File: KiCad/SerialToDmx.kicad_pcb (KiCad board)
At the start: 4 copper layers, 158 x 54 mm, 39 parts, among them J1 NAC3MPXXA, J10 Conn_01x08_Pin, J11 Conn_01x08_Pin, J2 NAC3MPXXB, J3 NC3FAV, J4 NC3MAV, J5 NC4FAV, J6 Conn_01x08_Socket, J7 Conn_01x08_Socket, J8 Conn_01x08_Pin, J9 Conn_01x08_Pin, U1 XIAO ESP32 C3, U2 ISOM8710DFFR, U3 ISOM8710DFFR, U4 ISOM8710DFFR, U5 THVD1512DGS, U6 SN74LV1T34DBV

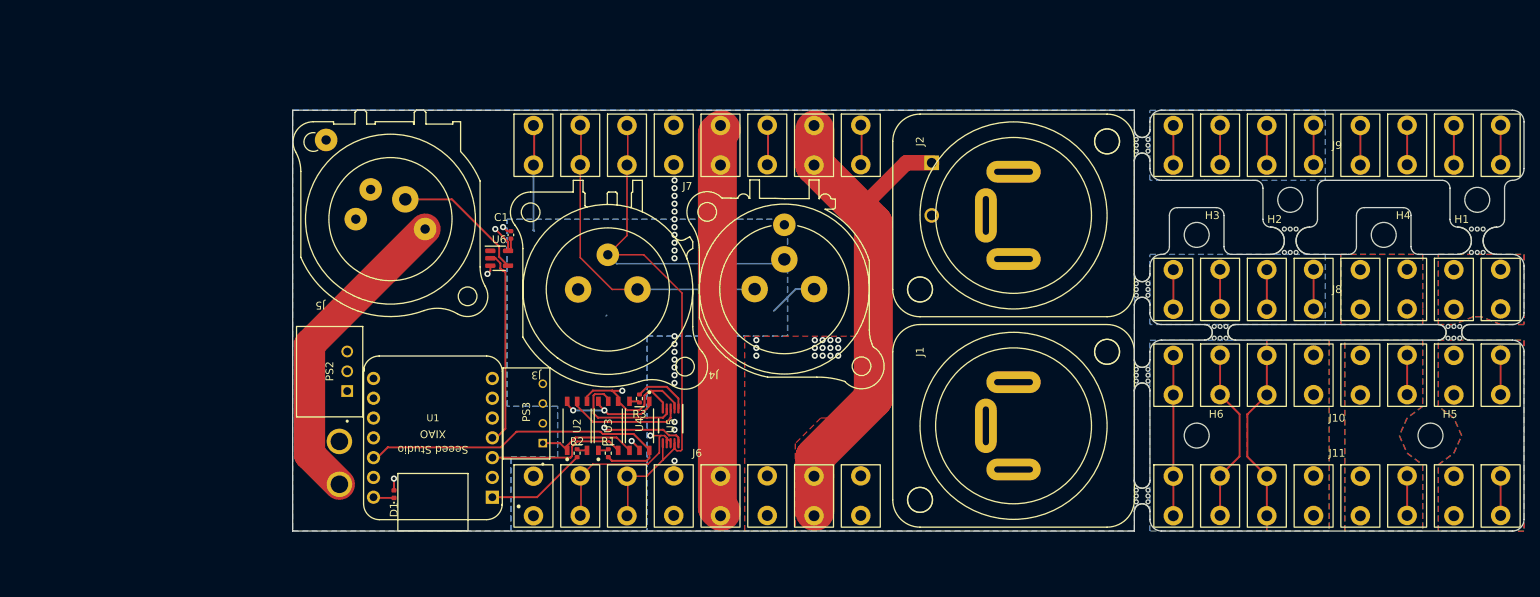
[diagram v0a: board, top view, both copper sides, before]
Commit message: With Files
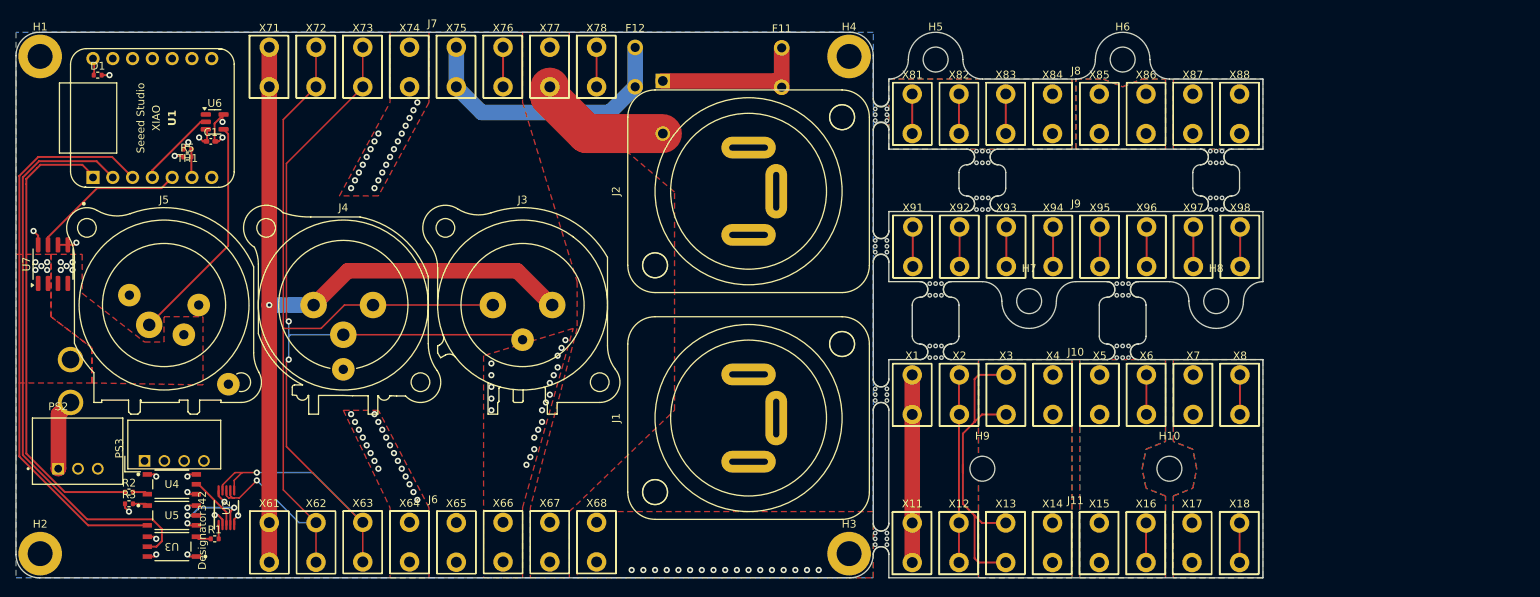
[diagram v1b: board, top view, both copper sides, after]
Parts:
- removed the H6 at (206.5, 106.8)
- added F11: 01110501Z, Custom_Littlefuse:fuseholder_111_501_Part1, F.Cu at (153.2, 59.5)
- added F12: 01110501Z, Custom_Littlefuse:fuseholder_111_501_Part2, F.Cu at (134.4, 59.5)
- added H10: MountingHole, MountingHole:MountingHole_3.2mm_M3, F.Cu at (203.0, 111.0)
- added H19: MountingHole, Panelization:mouse-bite-2mm-slot, F.Cu at (209.0, 71.0)
- added H20: MountingHole, Panelization:mouse-bite-2mm-slot, F.Cu at (209.0, 77.0)
- added H21: MountingHole, Panelization:mouse-bite-2mm-slot, F.Cu at (179.0, 71.0)
- added H22: MountingHole, Panelization:mouse-bite-2mm-slot, F.Cu at (179.0, 77.0)
- added H4: MountingHole_Pad, MountingHole:MountingHole_3.2mm_M3_DIN965_Pad, F.Cu at (161.9, 58.1)
- added H5: MountingHole, MountingHole:MountingHole_3.2mm_M3, F.Cu at (173.0, 58.5)
- added H8: MountingHole, MountingHole:MountingHole_3.2mm_M3, F.Cu at (209.0, 89.5)
- added H9: MountingHole, MountingHole:MountingHole_3.2mm_M3, F.Cu at (179.0, 111.0)
- added R5: 10kR, Resistor_SMD:R_0402_1005Metric, F.Cu at (77.0, 71.0)
- added TH1: Thermistor_PTC, Resistor_SMD:R_0402_1005Metric, F.Cu at (77.0, 70.0)
- added U7: NSM2012, Package_SO:SOIC-8_3.9x4.9mm_P1.27mm, F.Cu at (59.8, 84.8)
- added X1: 1217861-1, Custom_Connector_Faston:Faston_01x01_pin, F.Cu at (170.0, 101.5)
- added X11: 1217861-1, Custom_Connector_Faston:Faston_01x01_pin, F.Cu at (170.0, 120.5)
- added X12: 1217861-1, Custom_Connector_Faston:Faston_01x01_pin, F.Cu at (176.0, 120.5)
- added X13: 1217861-1, Custom_Connector_Faston:Faston_01x01_pin, F.Cu at (182.0, 120.5)
- added X14: 1217861-1, Custom_Connector_Faston:Faston_01x01_pin, F.Cu at (188.0, 120.5)
- added X15: 1217861-1, Custom_Connector_Faston:Faston_01x01_pin, F.Cu at (194.0, 120.5)
- added X16: 1217861-1, Custom_Connector_Faston:Faston_01x01_pin, F.Cu at (200.0, 120.5)
- added X17: 1217861-1, Custom_Connector_Faston:Faston_01x01_pin, F.Cu at (205.9, 120.5)
- added X18: 1217861-1, Custom_Connector_Faston:Faston_01x01_pin, F.Cu at (212.0, 120.5)
- added X2: 1217861-1, Custom_Connector_Faston:Faston_01x01_pin, F.Cu at (176.1, 101.5)
- added X3: 1217861-1, Custom_Connector_Faston:Faston_01x01_pin, F.Cu at (182.1, 101.5)
- added X4: 1217861-1, Custom_Connector_Faston:Faston_01x01_pin, F.Cu at (188.1, 101.5)
- added X5: 1217861-1, Custom_Connector_Faston:Faston_01x01_pin, F.Cu at (194.1, 101.5)
- added X6: 1217861-1, Custom_Connector_Faston:Faston_01x01_pin, F.Cu at (200.1, 101.5)
- added X61: 63994-1, Custom_Connector_Faston:Faston_01x01_socket, F.Cu at (87.5, 120.5)
- added X62: 63994-1, Custom_Connector_Faston:Faston_01x01_socket, F.Cu at (93.5, 120.5)
- added X63: 63994-1, Custom_Connector_Faston:Faston_01x01_socket, F.Cu at (99.5, 120.4)
- added X64: 63994-1, Custom_Connector_Faston:Faston_01x01_socket, F.Cu at (105.5, 120.4)
- added X65: 63994-1, Custom_Connector_Faston:Faston_01x01_socket, F.Cu at (111.5, 120.5)
- added X66: 63994-1, Custom_Connector_Faston:Faston_01x01_socket, F.Cu at (117.5, 120.4)
- added X67: 63994-1, Custom_Connector_Faston:Faston_01x01_socket, F.Cu at (123.5, 120.4)
- added X68: 63994-1, Custom_Connector_Faston:Faston_01x01_socket, F.Cu at (129.5, 120.4)
- added X7: 1217861-1, Custom_Connector_Faston:Faston_01x01_pin, F.Cu at (206.1, 101.5)
- added X71: 63994-1, Custom_Connector_Faston:Faston_01x01_socket, F.Cu at (87.5, 59.5)
- added X72: 63994-1, Custom_Connector_Faston:Faston_01x01_socket, F.Cu at (93.5, 59.5)
- added X73: 63994-1, Custom_Connector_Faston:Faston_01x01_socket, F.Cu at (99.5, 59.5)
- added X74: 63994-1, Custom_Connector_Faston:Faston_01x01_socket, F.Cu at (105.5, 59.5)
- added X75: 63994-1, Custom_Connector_Faston:Faston_01x01_socket, F.Cu at (111.5, 59.5)
- added X76: 63994-1, Custom_Connector_Faston:Faston_01x01_socket, F.Cu at (117.5, 59.5)
- added X77: 63994-1, Custom_Connector_Faston:Faston_01x01_socket, F.Cu at (123.5, 59.5)
- added X78: 63994-1, Custom_Connector_Faston:Faston_01x01_socket, F.Cu at (129.5, 59.5)
- added X8: 1217861-1, Custom_Connector_Faston:Faston_01x01_pin, F.Cu at (212.1, 101.5)
- added X81: 1217861-1, Custom_Connector_Faston:Faston_01x01_pin, F.Cu at (170.0, 65.5)
- added X82: 1217861-1, Custom_Connector_Faston:Faston_01x01_pin, F.Cu at (176.0, 65.5)
- added X83: 1217861-1, Custom_Connector_Faston:Faston_01x01_pin, F.Cu at (182.0, 65.5)
- added X84: 1217861-1, Custom_Connector_Faston:Faston_01x01_pin, F.Cu at (188.0, 65.5)
- added X85: 1217861-1, Custom_Connector_Faston:Faston_01x01_pin, F.Cu at (194.0, 65.5)
- added X86: 1217861-1, Custom_Connector_Faston:Faston_01x01_pin, F.Cu at (200.0, 65.5)
- added X87: 1217861-1, Custom_Connector_Faston:Faston_01x01_pin, F.Cu at (206.0, 65.5)
- added X88: 1217861-1, Custom_Connector_Faston:Faston_01x01_pin, F.Cu at (212.0, 65.5)
- added X91: 1217861-1, Custom_Connector_Faston:Faston_01x01_pin, F.Cu at (170.1, 82.5)
- added X92: 1217861-1, Custom_Connector_Faston:Faston_01x01_pin, F.Cu at (176.1, 82.5)
- added X93: 1217861-1, Custom_Connector_Faston:Faston_01x01_pin, F.Cu at (182.1, 82.5)
- added X94: 1217861-1, Custom_Connector_Faston:Faston_01x01_pin, F.Cu at (188.1, 82.5)
- added X95: 1217861-1, Custom_Connector_Faston:Faston_01x01_pin, F.Cu at (194.1, 82.5)
- added X96: 1217861-1, Custom_Connector_Faston:Faston_01x01_pin, F.Cu at (200.1, 82.5)
- added X97: 1217861-1, Custom_Connector_Faston:Faston_01x01_pin, F.Cu at (206.1, 82.5)
- added X98: 1217861-1, Custom_Connector_Faston:Faston_01x01_pin, F.Cu at (212.1, 82.5)
- C1: value 0.1uC -> 100nF; footprint Capacitor_SMD:C_0402_1005Metric -> Capacitor_SMD:C_0402_1005Metric_Pad0.74x0.62mm_HandSolder
- D1: value 1N4005 -> D; footprint Diode_SMD:D_0402_1005Metric -> Resistor_SMD:R_0402_1005Metric
- H1: value MountingHole -> MountingHole_Pad; footprint MountingHole:MountingHole_3.2mm_M3 -> MountingHole:MountingHole_3.2mm_M3_DIN965_Pad
- H11: renamed from H7; value Mousebite -> MountingHole
- H12: renamed from H8; value Mousebite -> MountingHole
- H13: renamed from H9; value Mousebite -> MountingHole
- H14: renamed from H10; value Mousebite -> MountingHole
- H15: renamed from H11; value Mousebite -> MountingHole
- H16: renamed from H12; value Mousebite -> MountingHole; footprint Panelization:mouse-bite-3.5mm-slot -> Panelization:mouse-bite-2mm-slot
- H17: renamed from H13; value Mousebite -> MountingHole; footprint Panelization:mouse-bite-3.5mm-slot -> Panelization:mouse-bite-2mm-slot
- H18: renamed from H14; value Mousebite -> MountingHole
- H2: renamed from H3; value MountingHole -> MountingHole_Pad; footprint MountingHole:MountingHole_3.2mm_M3 -> MountingHole:MountingHole_3.2mm_M3_DIN965_Pad
- H3: renamed from H5; value MountingHole -> MountingHole_Pad; footprint MountingHole:MountingHole_3.2mm_M3 -> MountingHole:MountingHole_3.2mm_M3_DIN965_Pad
- J1: footprint NeutrikCustom:NAC3MPXXA -> Custom_Neutrik:NAC3MPXXA
- J10, J11, J8, J9: value Conn_01x08_Pin -> ~; footprint Connector_Faston_Custom:Faston_01x08_pin -> Custom_Connector_Faston:Faston_01x08_pin
- J2: footprint NeutrikCustom:NAC3MPXXB -> Custom_Neutrik:NAC3MPXXB
- J3: footprint NeutrikCustom:NC3FAV -> Connector_Audio:Jack_XLR_Neutrik_NC3FAV_Vertical
- J4: footprint NeutrikCustom:NC3MAV -> Connector_Audio:Jack_XLR_Neutrik_NC3MAV_Vertical
- J5: footprint NeutrikCustom:NC4FAV -> Connector_Audio:Jack_XLR_Neutrik_NC4FAV_Vertical
- J6, J7: value Conn_01x08_Socket -> ~; footprint Connector_Faston_Custom:Faston_01x08_socket -> Custom_Connector_Faston:Faston_01x08_socket
- PS1: footprint IRM-45-12:CONV_IRM-45-12 -> Custom_Meanwell:CONV_IRM-45-12
- PS2: footprint CONV_R-78E5.0-0.5:CONV_R-78E5.0-0.5 -> Custom_Recom:CONV_R-78E5.0-0.5
- PS3: footprint TracoCustom:CONV_TEA_1-0505 -> Converter_DCDC:Converter_DCDC_TRACO_TEA1-xxxx_THT
- U2: renamed from U5; footprint TICustom:DGS0010A_N -> Custom_TI:DGS0010A_N
- U3: renamed from U4; footprint TICustom:ISOM8710 -> Custom_TI:ISOM8710
- U4: renamed from U2; footprint TICustom:ISOM8710 -> Custom_TI:ISOM8710
- U5: renamed from U3; footprint TICustom:ISOM8710 -> Custom_TI:ISOM8710
- moved H1 185.3 mm to (58.1, 58.1)
- moved H2 153.9 mm to (58.1, 121.9)
- moved H3 76.1 mm to (161.9, 121.9)
- moved H17 70.9 mm to (173.0, 96.0)
- moved D1 65.8 mm to (65.5, 60.5), turned to 0 degrees
- moved U3 62.0 mm to (75.0, 121.0), turned to 180 degrees
- moved R3 61.8 mm to (69.5, 115.5), turned to 0 degrees
- moved J4 60.3 mm to (93.2, 90.0), turned to 0 degrees
- moved U2 58.0 mm to (82.0, 116.0), turned to 90 degrees
- moved R2 57.7 mm to (69.5, 114.0), turned to 0 degrees
- moved R1 57.4 mm to (80.5, 120.0), turned to 0 degrees
- moved U5 57.2 mm to (75.0, 117.0), turned to 0 degrees
- moved U1 54.6 mm to (72.5, 66.0), turned to 90 degrees
- moved U4 52.5 mm to (75.0, 113.0), turned to 0 degrees
- moved PS3 51.5 mm to (71.5, 110.0)
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- renumbered H2 to H6, H4 to H7, R3 to R1, R1 to R3
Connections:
- J5 pad 2: GND -> LED-GND
- PS1 pad AC/L: L -> L-Fused
- U1 pad 5: unconnected-(U1-D4-Pad5) -> LED-Current-Sensor
- U1 pad 6: unconnected-(U1-D5-Pad6) -> Temperature Sensor
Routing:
- net N: track 128.5 -> 17.7 mm
- net GND: track 113.6 -> 8.70 mm, vias 23 -> 50
- net L: track 122.2 -> 35.9 mm
- net GND_Iso: track 40.9 -> 110.9 mm, vias 1 -> 5
- net DMX_TX: track 17.7 -> 72.7 mm
- net DMX_RX: track 20.9 -> 74.4 mm, vias 1 -> 0
- net DMX_DRIVE: track 12.5 -> 60.1 mm
- net Net-(X13-Pad1): track 0.00 -> 42.5 mm
- net 3V3: track 43.9 -> 2.47 mm, vias 0 -> 2
- net DMX+: track 89.8 -> 129.5 mm, vias 0 -> 3
- net 12V: track 85.8 -> 48.2 mm
- net DMX-: track 84.2 -> 115.5 mm
- net Net-(X1-Pad1): track 0.00 -> 24.1 mm
- net Net-(X12-Pad1): track 0.00 -> 24.1 mm
- net Net-(J10-Pin_3): track 22.7 -> 0.00 mm
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- added copper zone on In2.Cu, net 3V3
- added copper zone on In1.Cu, net 5V
- added copper zone on F.Cu, net GND
- added copper zone on In1.Cu, net GND
- added copper zone on In2.Cu, net GND
- added copper zone on F.Cu, net GND-Connection-In-Termination
- added copper zone on In2.Cu, net GND_Iso
- added copper zone on In1.Cu, net L
- added copper zone on In2.Cu, net L
- added copper zone on F.Cu, net L-switched
- added copper zone on F.Cu, net LED-GND
- added copper zone on In2.Cu, net LED-GND
- added copper zone on F.Cu, net N
- added copper zone on In1.Cu, net N
- added copper zone on In1.Cu, net VCC_Iso
- removed copper zone on In2.Cu, net 5V
- removed copper zone on B.Cu, net GND-Connection-Out-Termination
- removed copper zone on In1.Cu, net GND-Connection-Out-Termination
- removed copper zone on In2.Cu, net GND-Connection-Out-Termination
- removed copper zone on B.Cu, net GND_Iso
- removed copper zone on In2.Cu, net N-switched
- removed copper zone on In2.Cu, net VCC_Iso
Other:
- board size 158 x 54 mm -> 160 x 70 mm
